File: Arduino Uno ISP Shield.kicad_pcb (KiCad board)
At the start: 2 copper layers, 68.6 x 53.3 mm, 30 parts, among them J1 CONN_POWER, J10 Conn_01x01_Female, J2 CONN_ANALOG_IN, J3 Conn_01x02_Male, J34 CONN_DIGITAL_8-13, J35 CONN_DIGITAL_0-7, J4 Conn_02x03_Odd_Even, J5 Conn_01x01_Female, J6 Conn_01x01_Female, J7 Conn_01x01_Female, J8 Conn_01x01_Female, J9 Conn_01x01_Female, U1 ATmega328P-PU

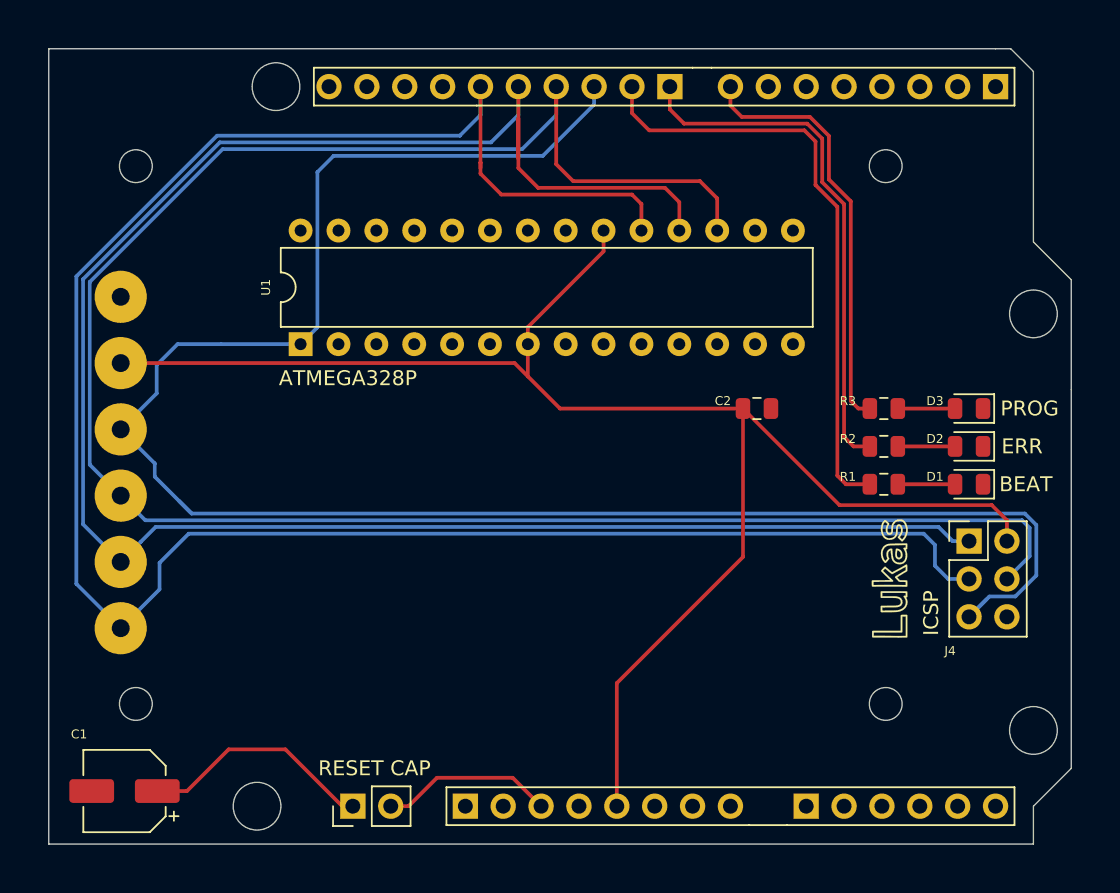
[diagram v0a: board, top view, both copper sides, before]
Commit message: Add fabrication data
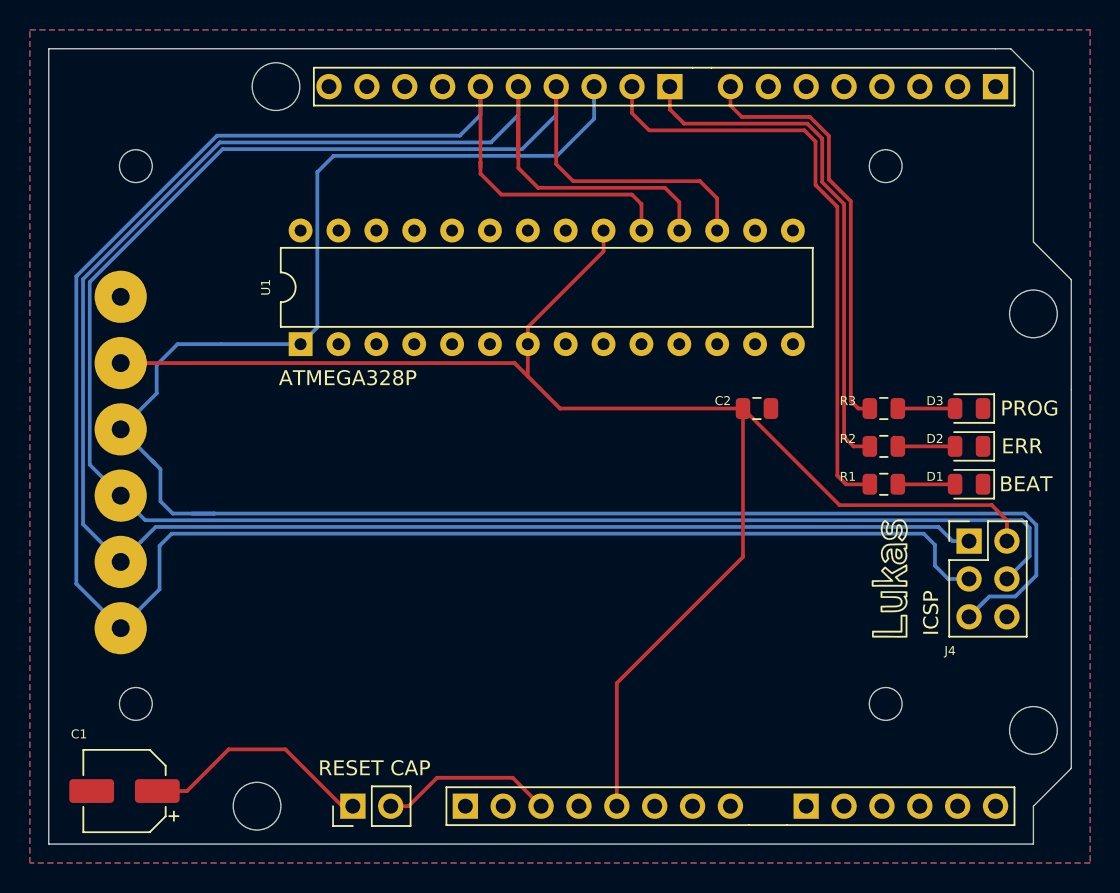
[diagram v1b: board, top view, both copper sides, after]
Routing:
- net ICSP_RST: track 125.6 -> 127.6 mm
- net ICSP_SCK: track 140.6 -> 141.3 mm
- added copper zone on B.Cu, net GND
- added copper zone on F.Cu, net GND
